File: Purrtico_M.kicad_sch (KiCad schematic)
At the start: 93 parts, among them J1 Conn_02x05_Odd_Even, J2 Conn_01x02, J4 Conn_01x02, U1 OPA1679, U2 OPA1679, U3 OPA1679

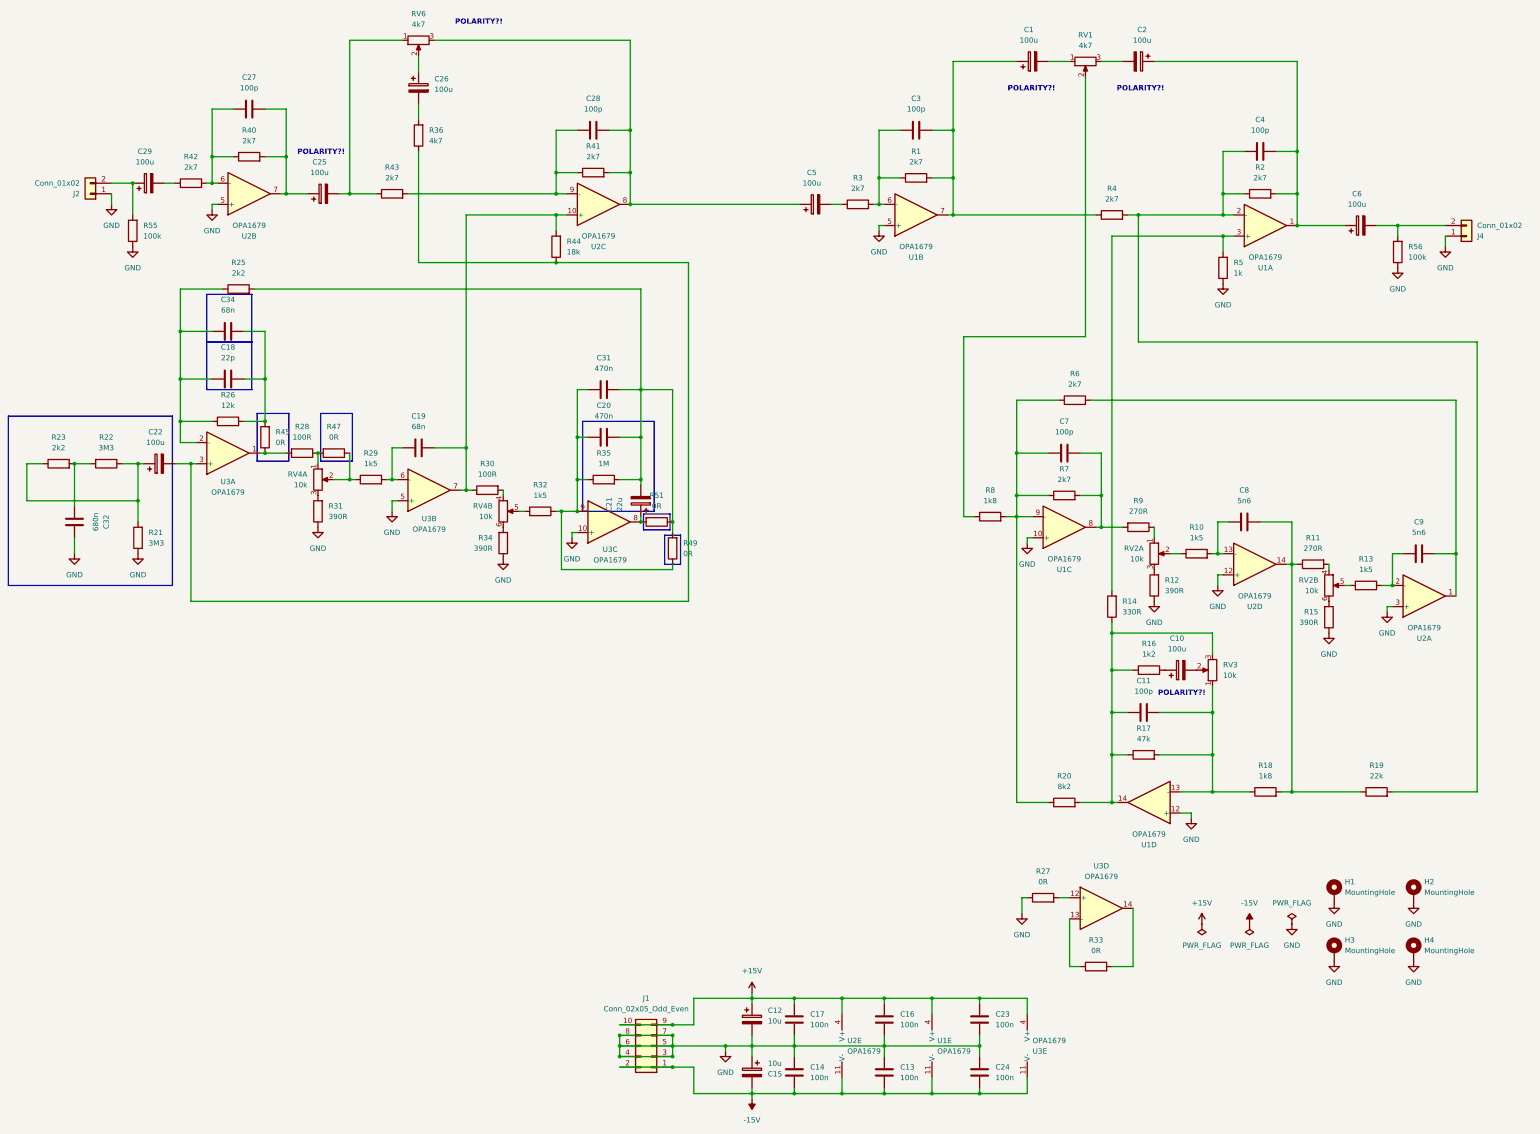
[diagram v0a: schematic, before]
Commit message: whatever
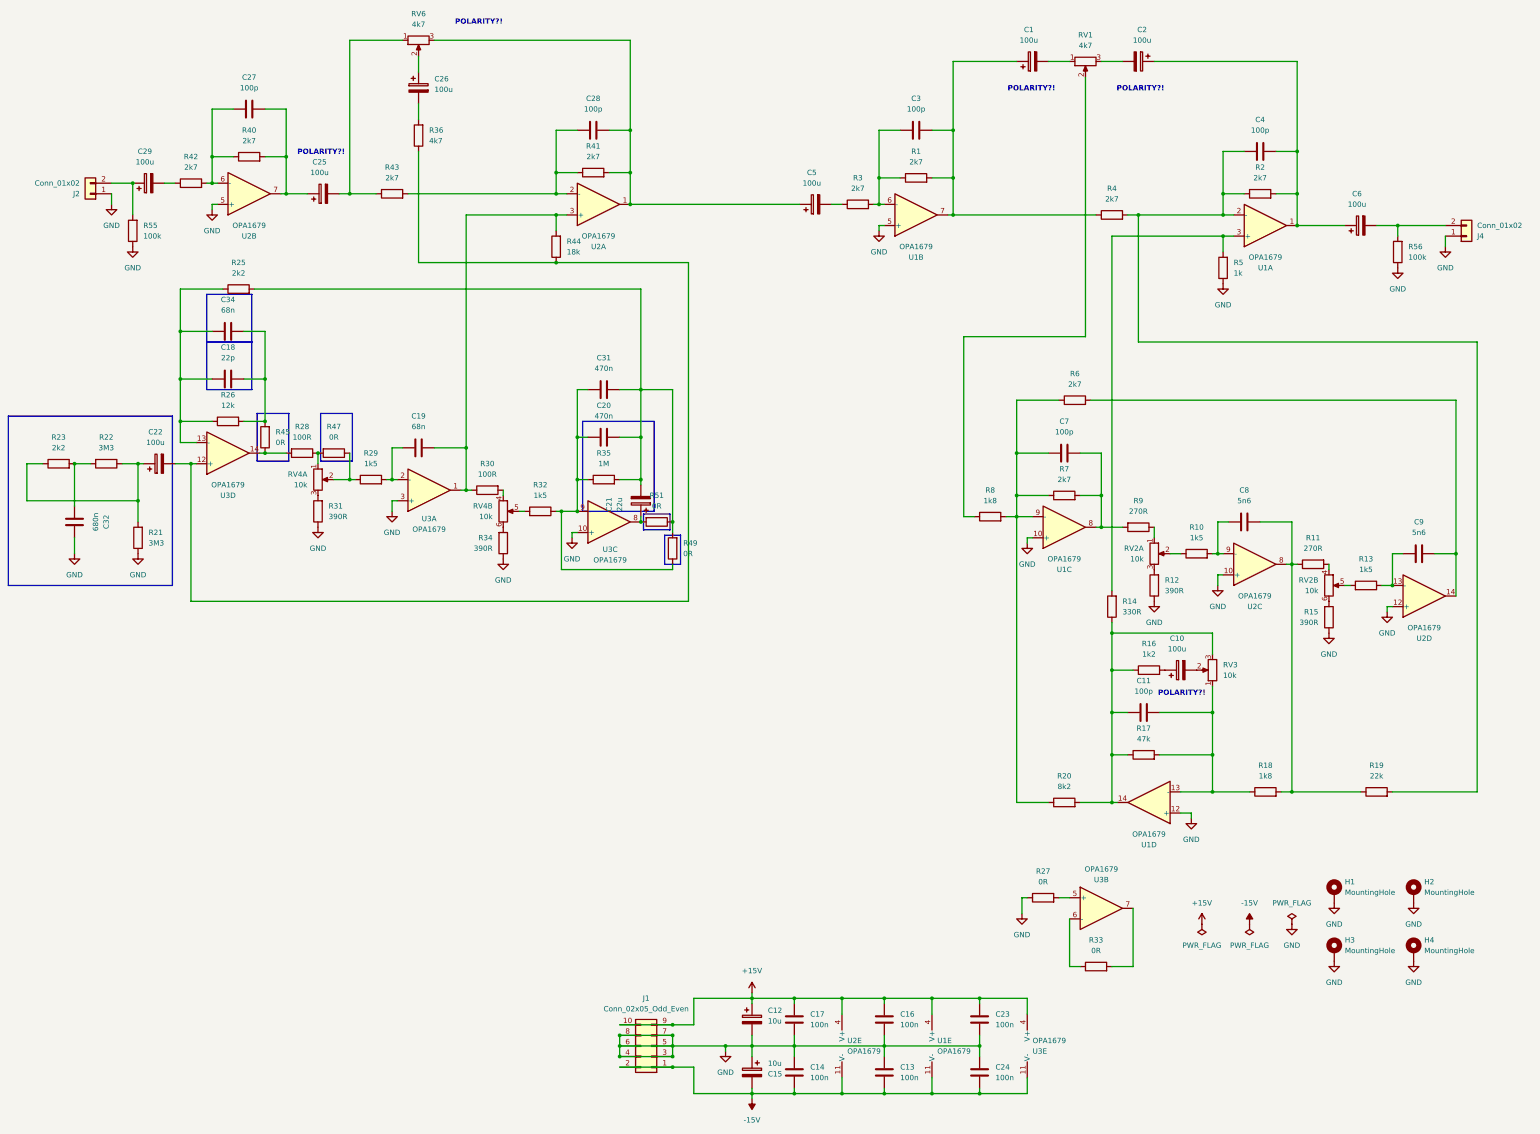
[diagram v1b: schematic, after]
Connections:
- net GND: now also U2.10 (+), U3.3 (+); no longer U2.3 (+), U3.5 (+)
- net at C18.1, C34.1, R25.1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: now also U3.13 (-); no longer U3.2 (-)
- net at C19.1, R29.2: now also U3.2 (-); no longer U3.6 (-)
- net at C19.2, R30.1, R44.2: now also U2.3 (+), U3.1; no longer U2.10 (+), U3.7
- net at R27.2: now also U3.5 (+); no longer U3.12 (+)
- net at C28.1, R41.1, R43.2: now also U2.2 (-); no longer U2.9 (-)
- net at R28.2, R45.1: now also U3.14; no longer U3.1
- net at C28.2, C5.1, R41.2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: now also U2.1; no longer U2.8
- net at C9.2, R6.2: now also U2.14; no longer U2.1
- net at C9.1, R13.1: now also U2.13 (-); no longer U2.2 (-)
- net at C8.1, R10.2: now also U2.9 (-); no longer U2.13 (-)
- net at C8.2, R11.1, R18.2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: now also U2.8; no longer U2.14
- net at C22.2, R36.1, R44.1: now also U3.12 (+); no longer U3.3 (+)
- net at R33.1: now also U3.6 (-); no longer U3.13 (-)
- net at R33.2: now also U3.7; no longer U3.14
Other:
- moved on the sheet: U2A, U2C, U2D, U3A, U3B, U3D
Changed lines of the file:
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@@
 	)
 	(junction
+		(at 186.69 62.23)
+		(diameter 0)
+		(color 0 0 0 0)
+	)
+	(junction
 		(at 264.16 44.45)
 		(diameter 0)
@@
 	)
 	(junction
-		(at 369.57 153.67)
-		(diameter 0)
-		(color 0 0 0 0)
-	)
-	(junction
 		(at 328.93 59.69)
 		(diameter 0)
@@
 	)
 	(junction
-		(at 186.69 62.23)
+		(at 196.85 259.08)
 		(diameter 0)
 		(color 0 0 0 0)
 	)
 	(junction
-		(at 196.85 259.08)
+		(at 168.91 59.69)
 		(diameter 0)
 		(color 0 0 0 0)
 	)
 	(junction
-		(at 168.91 59.69)
+		(at 173.99 128.27)
 		(diameter 0)
 		(color 0 0 0 0)
 	)
 	(junction
-		(at 173.99 128.27)
+		(at 369.57 153.67)
 		(diameter 0)
 		(color 0 0 0 0)
@@
 	(symbol
 		(lib_id "Amplifier_Operational:OPA1679")
-		(at 179.07 62.23 0)
+		(at 336.55 148.59 0)
 		(mirror x)
 		(unit 3)
@@
 		(dnp no)
 		(property "Reference" "U2"
-			(at 179.07 72.39 0)
+			(at 336.55 158.75 0)
 			(effects
 				(font
@@
 		)
 		(property "Value" "OPA1679"
-			(at 179.07 69.85 0)
+			(at 336.55 156.21 0)
 			(effects
 				(font
@@
 		)
 		(property "Footprint" "Package_SO:SOIC-14_3.9x8.7mm_P1.27mm"
-			(at 177.8 64.77 0)
+			(at 335.28 151.13 0)
 			(effects
 				(font
@@
 		)
 		(property "Datasheet" "http://www.ti.com/lit/ds/symlink/opa1678.pdf"
-			(at 180.34 67.31 0)
+			(at 337.82 153.67 0)
 			(effects
 				(font
@@
 		)
 		(property "Description" "Low-Distortion Audio Operational Amplifiers, SOIC-14/TSSOP-14"
-			(at 179.07 62.23 0)
+			(at 336.55 148.59 0)
 			(effects
 				(font
@@
 	(symbol
 		(lib_id "Amplifier_Operational:OPA1679")
-		(at 377.19 156.21 0)
+		(at 179.07 62.23 0)
 		(mirror x)
 		(unit 1)
@@
 		(dnp no)
 		(property "Reference" "U2"
-			(at 377.19 166.37 0)
+			(at 179.07 72.39 0)
 			(effects
 				(font
@@
 		)
 		(property "Value" "OPA1679"
-			(at 377.19 163.83 0)
+			(at 179.07 69.85 0)
 			(effects
 				(font
@@
 		)
 		(property "Footprint" "Package_SO:SOIC-14_3.9x8.7mm_P1.27mm"
-			(at 375.92 158.75 0)
+			(at 177.8 64.77 0)
 			(effects
 				(font
@@
 		)
 		(property "Datasheet" "http://www.ti.com/lit/ds/symlink/opa1678.pdf"
-			(at 378.46 161.29 0)
+			(at 180.34 67.31 0)
 			(effects
 				(font
@@
 		)
 		(property "Description" "Low-Distortion Audio Operational Amplifiers, SOIC-14/TSSOP-14"
-			(at 377.19 156.21 0)
+			(at 179.07 62.23 0)
 			(effects
 				(font
@@
 	(symbol
 		(lib_id "Amplifier_Operational:OPA1679")
-		(at 90.17 121.92 0)
+		(at 138.43 130.81 0)
 		(mirror x)
 		(unit 1)
@@
 		(dnp no)
 		(property "Reference" "U3"
-			(at 90.17 128.778 0)
+			(at 138.43 137.668 0)
 			(effects
 				(font
@@
 		)
 		(property "Value" "OPA1679"
-			(at 90.17 131.318 0)
+			(at 138.43 140.208 0)
 			(effects
 				(font
@@
 		)
 		(property "Footprint" "Package_SO:SOIC-14_3.9x8.7mm_P1.27mm"
-			(at 88.9 124.46 0)
+			(at 137.16 133.35 0)
 			(effects
 				(font
@@
 		)
 		(property "Datasheet" "http://www.ti.com/lit/ds/symlink/opa1678.pdf"
-			(at 91.44 127 0)
+			(at 139.7 135.89 0)
 			(effects
 				(font
@@
 		)
 		(property "Description" "Low-Distortion Audio Operational Amplifiers, SOIC-14/TSSOP-14"
-			(at 90.17 121.92 0)
+			(at 138.43 130.81 0)
 			(effects
 				(font
@@
 	(symbol
 		(lib_id "Amplifier_Operational:OPA1679")
-		(at 138.43 130.81 0)
-		(mirror x)
+		(at 299.72 231.14 0)
 		(unit 2)
 		(exclude_from_sim no)
@@
 		(dnp no)
 		(property "Reference" "U3"
-			(at 138.43 137.668 0)
+			(at 299.72 224.282 0)
 			(effects
 				(font
@@
 		)
 		(property "Value" "OPA1679"
-			(at 138.43 140.208 0)
+			(at 299.72 221.742 0)
 			(effects
 				(font
@@
 		)
 		(property "Footprint" "Package_SO:SOIC-14_3.9x8.7mm_P1.27mm"
-			(at 137.16 133.35 0)
+			(at 298.45 228.6 0)
 			(effects
 				(font
@@
 		)
 		(property "Datasheet" "http://www.ti.com/lit/ds/symlink/opa1678.pdf"
-			(at 139.7 135.89 0)
+			(at 300.99 226.06 0)
 			(effects
 				(font
@@
 		)
 		(property "Description" "Low-Distortion Audio Operational Amplifiers, SOIC-14/TSSOP-14"
-			(at 138.43 130.81 0)
+			(at 299.72 231.14 0)
 			(effects
 				(font
@@
 	(symbol
 		(lib_id "Amplifier_Operational:OPA1679")
-		(at 336.55 148.59 0)
+		(at 377.19 156.21 0)
 		(mirror x)
 		(unit 4)
@@
 		(dnp no)
 		(property "Reference" "U2"
-			(at 336.55 158.75 0)
+			(at 377.19 166.37 0)
 			(effects
 				(font
@@
 		)
 		(property "Value" "OPA1679"
-			(at 336.55 156.21 0)
+			(at 377.19 163.83 0)
 			(effects
 				(font
@@
 		)
 		(property "Footprint" "Package_SO:SOIC-14_3.9x8.7mm_P1.27mm"
-			(at 335.28 151.13 0)
+			(at 375.92 158.75 0)
 			(effects
 				(font
@@
 		)
 		(property "Datasheet" "http://www.ti.com/lit/ds/symlink/opa1678.pdf"
-			(at 337.82 153.67 0)
+			(at 378.46 161.29 0)
 			(effects
 				(font
@@
 		)
 		(property "Description" "Low-Distortion Audio Operational Amplifiers, SOIC-14/TSSOP-14"
-			(at 336.55 148.59 0)
+			(at 377.19 156.21 0)
 			(effects
 				(font
@@
 	(symbol
 		(lib_id "Amplifier_Operational:OPA1679")
-		(at 299.72 231.14 0)
+		(at 90.17 121.92 0)
+		(mirror x)
 		(unit 4)
 		(exclude_from_sim no)
@@
 		(dnp no)
 		(property "Reference" "U3"
-			(at 299.72 220.98 0)
+			(at 90.17 132.08 0)
 			(effects
 				(font
@@
 		)
 		(property "Value" "OPA1679"
-			(at 299.72 223.52 0)
+			(at 90.17 129.54 0)
 			(effects
 				(font
@@
 		)
 		(property "Footprint" "Package_SO:SOIC-14_3.9x8.7mm_P1.27mm"
-			(at 298.45 228.6 0)
+			(at 88.9 124.46 0)
 			(effects
 				(font
@@
 		)
 		(property "Datasheet" "http://www.ti.com/lit/ds/symlink/opa1678.pdf"
-			(at 300.99 226.06 0)
+			(at 91.44 127 0)
 			(effects
 				(font
@@
 		)
 		(property "Description" "Low-Distortion Audio Operational Amplifiers, SOIC-14/TSSOP-14"
-			(at 299.72 231.14 0)
+			(at 90.17 121.92 0)
 			(effects
 				(font
